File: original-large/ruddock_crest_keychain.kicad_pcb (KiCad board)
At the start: 2 copper layers, 50.8 x 50.8 mm, 10 parts

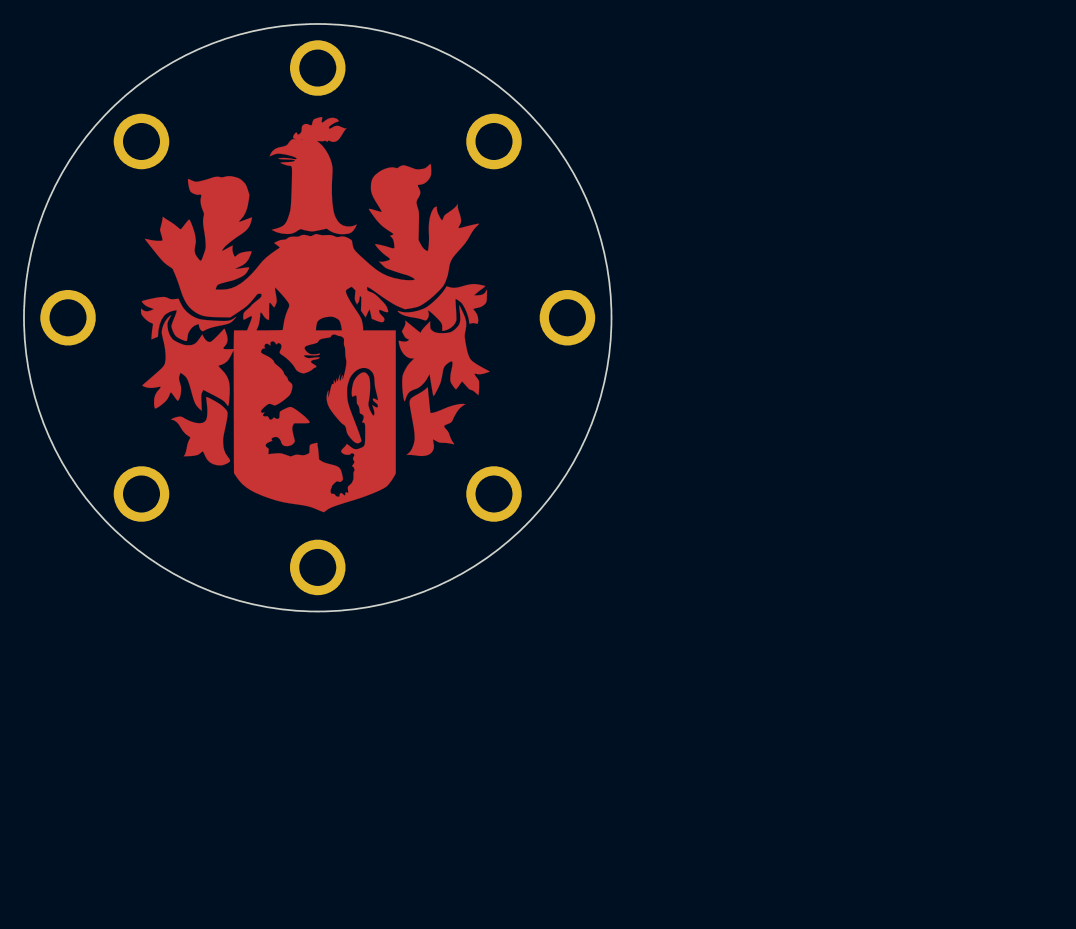
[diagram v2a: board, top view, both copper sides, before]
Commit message: Update title block
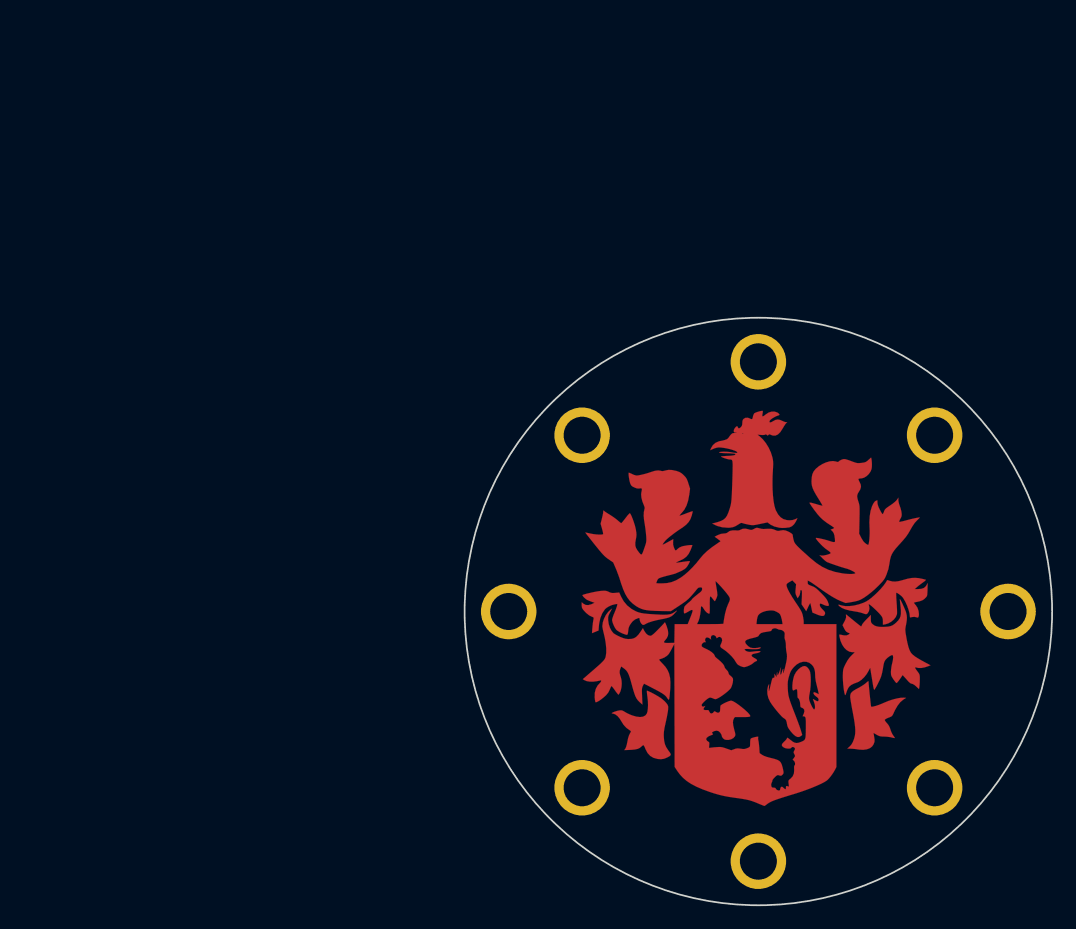
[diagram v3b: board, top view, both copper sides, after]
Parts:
- removed the REF** at (86.4, 91.4)
- removed the REF** at (116.8, 61.0)
- removed the REF** at (86.4, 61.0)
- removed the REF** at (101.6, 97.8)
- removed the REF** at (123.2, 76.2)
- added REF**: MountingHole_3.2mm_M3_Pad, MountingHole:MountingHole_3.2mm_M3_Pad, F.Cu at (124.5, 116.8)
- added REF**: MountingHole_3.2mm_M3_Pad, MountingHole:MountingHole_3.2mm_M3_Pad, F.Cu at (154.9, 86.4)
- added REF**: MountingHole_3.2mm_M3_Pad, MountingHole:MountingHole_3.2mm_M3_Pad, F.Cu at (124.5, 86.4)
- added REF**: MountingHole_3.2mm_M3_Pad, MountingHole:MountingHole_3.2mm_M3_Pad, F.Cu at (139.7, 123.2)
- added REF**: MountingHole_3.2mm_M3_Pad, MountingHole:MountingHole_3.2mm_M3_Pad, F.Cu at (161.3, 101.6)
- moved REF** 45.8 mm to (154.9, 116.8)
- moved REF** 45.8 mm to (139.7, 80.0)
- moved G*** 45.8 mm to (139.7, 101.6) (x2)
- moved REF** 45.8 mm to (118.1, 101.6)
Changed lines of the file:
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@@
     (nets 1)
   )
-  (page A4)
+  (page A)
+  (title_block
+    (title "Ruddock House PCB Crest")
+    (date 2019-01-24)
+    (rev A)
+    (company "Ruddock House Electrical Engineering")
+    (comment 1 "Ray Sun")
+  )
   (layers
     (0 F.Cu signal)
@@
     (solder_mask_min_width 0.25)
     (aux_axis_origin 0 0)
-    (grid_origin 76.2 101.6)
+    (grid_origin 114.3 127)
     (visible_elements 7FFFFFFF)
     (pcbplotparams
@@
   )
   (module MountingHole:MountingHole_3.2mm_M3_Pad (layer F.Cu)
-    (at 116.84 91.44)
+    (at 154.94 116.84)
     (descr "Mounting Hole 3.2mm, M3")
     (tags "mounting hole 3.2mm m3")
@@
   )
   (module MountingHole:MountingHole_3.2mm_M3_Pad (layer F.Cu)
-    (at 86.36 91.44)
+    (at 124.46 116.84)
     (descr "Mounting Hole 3.2mm, M3")
     (tags "mounting hole 3.2mm m3")
@@
   )
   (module MountingHole:MountingHole_3.2mm_M3_Pad (layer F.Cu)
-    (at 116.84 60.96)
+    (at 154.94 86.36)
     (descr "Mounting Hole 3.2mm, M3")
     (tags "mounting hole 3.2mm m3")
@@
   )
   (module MountingHole:MountingHole_3.2mm_M3_Pad (layer F.Cu)
-    (at 86.36 60.96)
+    (at 124.46 86.36)
     (descr "Mounting Hole 3.2mm, M3")
     (tags "mounting hole 3.2mm m3")
@@
   )
   (module MountingHole:MountingHole_3.2mm_M3_Pad (layer F.Cu)
-    (at 101.6 97.79)
+    (at 139.7 123.19)
     (descr "Mounting Hole 3.2mm, M3")
     (tags "mounting hole 3.2mm m3")
@@
   )
   (module MountingHole:MountingHole_3.2mm_M3_Pad (layer F.Cu)
-    (at 123.19 76.2)
+    (at 161.29 101.6)
     (descr "Mounting Hole 3.2mm, M3")
     (tags "mounting hole 3.2mm m3")
@@
   )
   (module MountingHole:MountingHole_3.2mm_M3_Pad (layer F.Cu)
-    (at 80.01 76.2)
+    (at 118.11 101.6)
     (descr "Mounting Hole 3.2mm, M3")
     (tags "mounting hole 3.2mm m3")
@@
   )
   (module crest:ruddock_cu (layer F.Cu)
-    (at 101.6 76.2)
+    (at 139.7 101.6)
     (fp_text reference G*** (at 0 0) (layer F.SilkS) hide
       (effects (font (size 1.524 1.524) (thickness 0.3)))
@@
   )
   (module crest:ruddock_mask (layer F.Cu)
-    (at 101.6 76.2)
+    (at 139.7 101.6)
     (fp_text reference G*** (at 0 0) (layer F.SilkS) hide
       (effects (font (size 1.524 1.524) (thickness 0.3)))
@@
   )
   (module MountingHole:MountingHole_3.2mm_M3_Pad (layer F.Cu)
-    (at 101.6 54.61)
+    (at 139.7 80.01)
     (descr "Mounting Hole 3.2mm, M3")
     (tags "mounting hole 3.2mm m3")
@@
     (pad 1 thru_hole circle (at 0 0) (size 4.8 4.8) (drill 3.2) (layers *.Cu *.Mask))
   )
-  (gr_text "VIRTUTIS\nMAMMAILAS\nEXSUGIMUS" (at 101.6 83.82) (layer B.SilkS)
+  (gr_text "VIRTUTIS\nMAMMAILAS\nEXSUGIMUS" (at 139.7 109.22) (layer B.SilkS)
     (effects (font (size 2.2 2.2) (thickness 0.5)) (justify mirror))
   )
-  (gr_text "PCB Crest" (at 101.6 73.66) (layer B.SilkS)
+  (gr_text "PCB Crest" (at 139.7 99.06) (layer B.SilkS)
     (effects (font (size 3 3) (thickness 0.6)) (justify mirror))
   )
-  (gr_text "Ruddock House" (at 101.6 68.58) (layer B.SilkS)
+  (gr_text "Ruddock House" (at 139.7 93.98) (layer B.SilkS)
     (effects (font (size 3 3) (thickness 0.6)) (justify mirror))
   )
-  (gr_circle (center 101.6 76.2) (end 101.6 50.8) (layer Edge.Cuts) (width 0.15))
+  (gr_circle (center 139.7 101.6) (end 139.7 76.2) (layer Edge.Cuts) (width 0.15))
 )
